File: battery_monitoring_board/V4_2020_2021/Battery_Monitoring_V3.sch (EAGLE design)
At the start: 116 parts, among them CON1 MOLEX_5566-2, CON2 SM03B-GHS-TB, CON3 SM03B-GHS-TB, J1 MKDS_5/2-6,352, J10 MKDS_5/2-6,352, J16 MKDS_5/2-6,352, J2 MKDS_5/2-6,352, J3 MKDS_5/2-6,352, J4 MKDS_5/2-6,352, J9 MKDS_5/2-6,352, Q1 TCLD1000CT, Q10 SI7145DP, Q11 SI7145DP, Q12 SI7145DP, Q13 SI7145DP, Q14 SI7145DP, Q15 PSMN1R5-30BLE, Q16 TCLD1000CT, Q17 NMOS-TO252, Q18 NMOS-TO252, Q19 NMOS-TO252, Q2 TCLD1000CT, Q20 NMOS-TO252, Q21 DMN2011UTS, Q3 TCLD1000CT, Q4 PSMN1R5-30BLE, Q5 PSMN1R5-30BLE, Q6 PSMN1R5-30BLE, Q7 SI7145DP, Q8 SI7145DP, Q9 SI7145DP, U1 INA3221., U10 LM5050-2, U12 IR2301S, U2 INA3221., U3 TEENSY_3.1_BASIC_2, U4 TCAN1042HVDR, U5 LTC4418, U6 LM5050-2, U7 LM5050-2, U8 LM5050-2

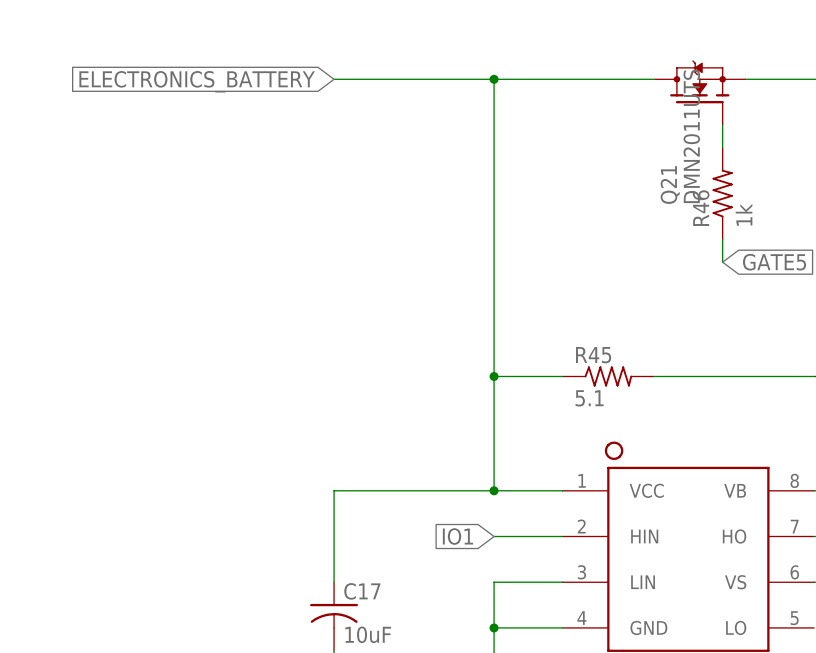
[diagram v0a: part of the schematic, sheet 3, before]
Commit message: started work on PCB layout
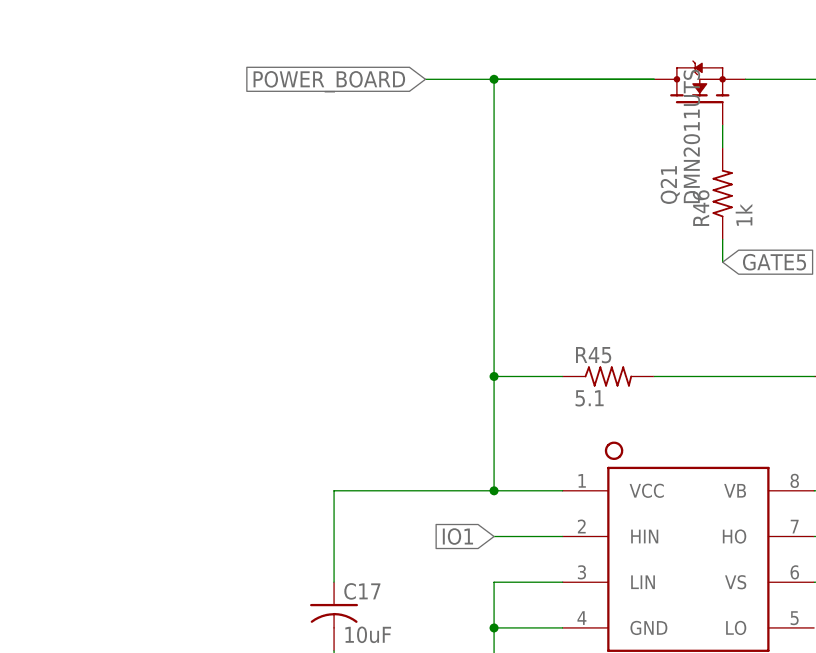
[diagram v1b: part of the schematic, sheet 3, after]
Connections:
- net ELECTRONICS_BATTERY: no longer C17.1, Q21.D, R45.1, U12.VCC
- net POWER_BOARD: now also C17.1, Q21.D, R45.1, U12.VCC
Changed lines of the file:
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@@
-</segment>
-</net>
-<net name="ELECTRONICS_BATTERY" class="0">
-<segment>
-<wire x1="-251.46" y1="63.5" x2="-233.68" y2="63.5" width="0.1524" layer="91"/>
-<wire x1="-233.68" y1="63.5" x2="-215.9" y2="63.5" width="0.1524" layer="91"/>
-<pinref part="Q21" gate="G$1" pin="D"/>
-<wire x1="-251.46" y1="7.62" x2="-251.46" y2="17.78" width="0.1524" layer="91"/>
-<pinref part="U12" gate="G$1" pin="VCC"/>
-<wire x1="-251.46" y1="17.78" x2="-233.68" y2="17.78" width="0.1524" layer="91"/>
-<wire x1="-233.68" y1="17.78" x2="-226.06" y2="17.78" width="0.1524" layer="91"/>
-<wire x1="-233.68" y1="63.5" x2="-233.68" y2="30.48" width="0.1524" layer="91"/>
-<junction x="-233.68" y="63.5"/>
-<junction x="-233.68" y="17.78"/>
-<pinref part="C17" gate="G$1" pin="1"/>
-<pinref part="R45" gate="G$1" pin="1"/>
-<wire x1="-233.68" y1="30.48" x2="-233.68" y2="17.78" width="0.1524" layer="91"/>
-<wire x1="-233.68" y1="30.48" x2="-226.06" y2="30.48" width="0.1524" layer="91"/>
-<junction x="-233.68" y="30.48"/>
-<label x="-251.46" y="63.5" size="1.778" layer="95" rot="R180" xref="yes"/>
 </segment>
 </net>
@@
 </segment>
 </net>
+<net name="POWER_BOARD" class="0">
+<segment>
+<pinref part="C17" gate="G$1" pin="1"/>
+<pinref part="U12" gate="G$1" pin="VCC"/>
+<wire x1="-251.46" y1="7.62" x2="-251.46" y2="17.78" width="0.1524" layer="91"/>
+<wire x1="-251.46" y1="17.78" x2="-233.68" y2="17.78" width="0.1524" layer="91"/>
+<wire x1="-226.06" y1="17.78" x2="-233.68" y2="17.78" width="0.1524" layer="91"/>
+<pinref part="R45" gate="G$1" pin="1"/>
+<wire x1="-233.68" y1="17.78" x2="-233.68" y2="30.48" width="0.1524" layer="91"/>
+<wire x1="-226.06" y1="30.48" x2="-233.68" y2="30.48" width="0.1524" layer="91"/>
+<pinref part="Q21" gate="G$1" pin="D"/>
+<wire x1="-233.68" y1="30.48" x2="-233.68" y2="63.5" width="0.1524" layer="91"/>
+<wire x1="-233.68" y1="63.5" x2="-215.9" y2="63.5" width="0.1524" layer="91"/>
+<wire x1="-215.9" y1="63.5" x2="-233.68" y2="63.5" width="0.1524" layer="91"/>
+<label x="-241.3" y="63.5" size="1.778" layer="95" rot="R180" xref="yes"/>
+<junction x="-233.68" y="63.5"/>
+<wire x1="-233.68" y1="63.5" x2="-241.3" y2="63.5" width="0.1524" layer="91"/>
+<junction x="-233.68" y="30.48"/>
+<junction x="-233.68" y="17.78"/>
+</segment>
+</net>
